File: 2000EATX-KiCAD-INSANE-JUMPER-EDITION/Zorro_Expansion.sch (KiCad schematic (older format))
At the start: 111 parts, among them CN601 Amiga-2000-Zorro-Slot, CN602 Amiga-2000-Zorro-Slot, CN603 Amiga-2000-Zorro-Slot, CN604 Amiga-2000-Zorro-Slot, CN605 Amiga-2000-Zorro-Slot, U606 74HCT32

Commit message: Add files via upload
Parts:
- C617, C619, C620, C621, C622, C623, C624, C625, C626, C627, C628, C629, C630, C631, C632, C633, C635, C637, C639, C641, C645, C647, C649, C650, C651, C652, C654, C655, C657, C658, C659, C660, C661, C662, C663, C664, C665, C666, C667, C668, C669, C670, C671, C672, C673, C674, C675: footprint Capacitor_SMD:C_1206_3216Metric -> Capacitor_SMD:C_0805_2012Metric
- R601A1, R601B1, R601C1, R601D1, R601E1, R601F1, R601G1, R601H1, R601I1, R602A1, R602B1, R602C1, R602D1, R602E1, R602F1, R602G1, R602H1, R602I1, R603A1, R603B1, R603C1, R603D1, R603E1, R603F1, R603G1, R603H1, R603I1, R604, R604A1, R604B1, R604C1, R604D1, R604E1, R604F1, R604G1, R604H1, R604I1, R605, R605A1, R605B1, R605C1, R605D1, R605E1, R605F1, R605G1, R605H1, R605I1: footprint Resistor_SMD:R_1206_3216Metric -> Resistor_SMD:R_0805_2012Metric

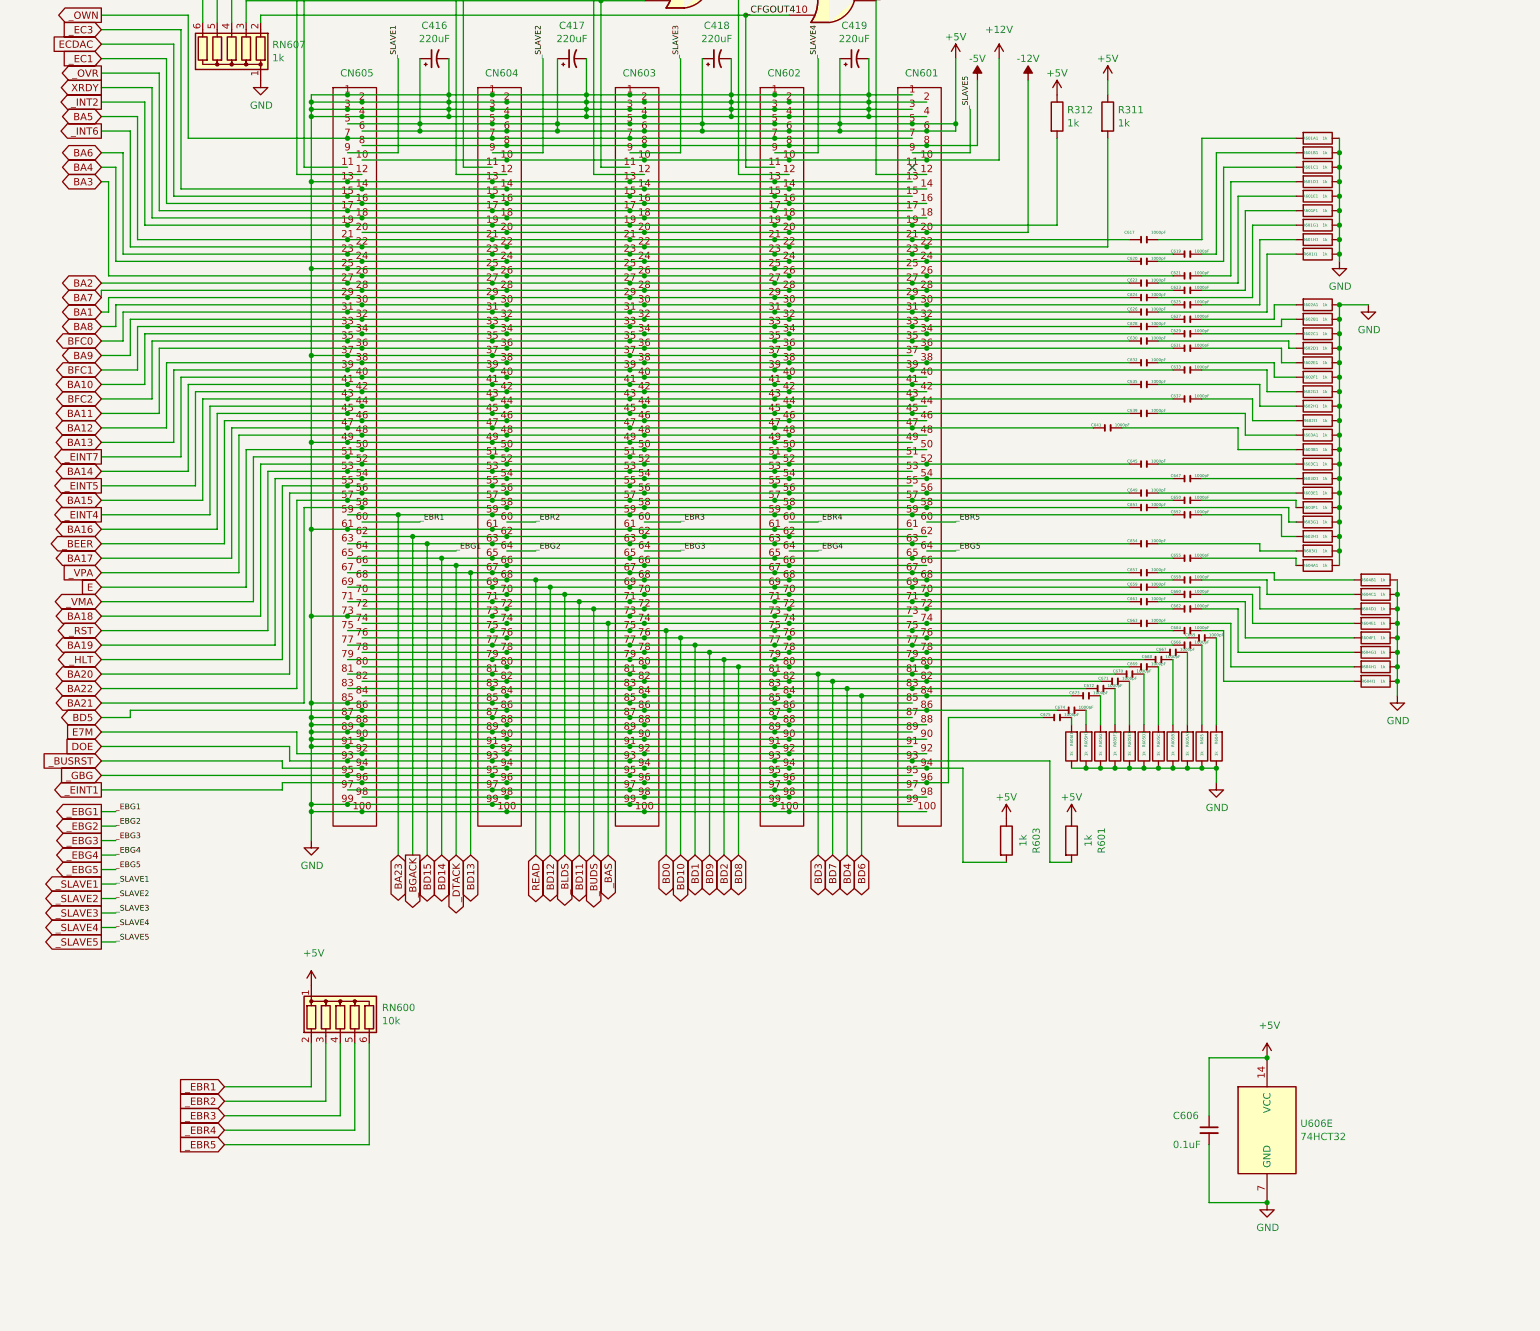
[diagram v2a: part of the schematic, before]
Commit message: Add files via upload
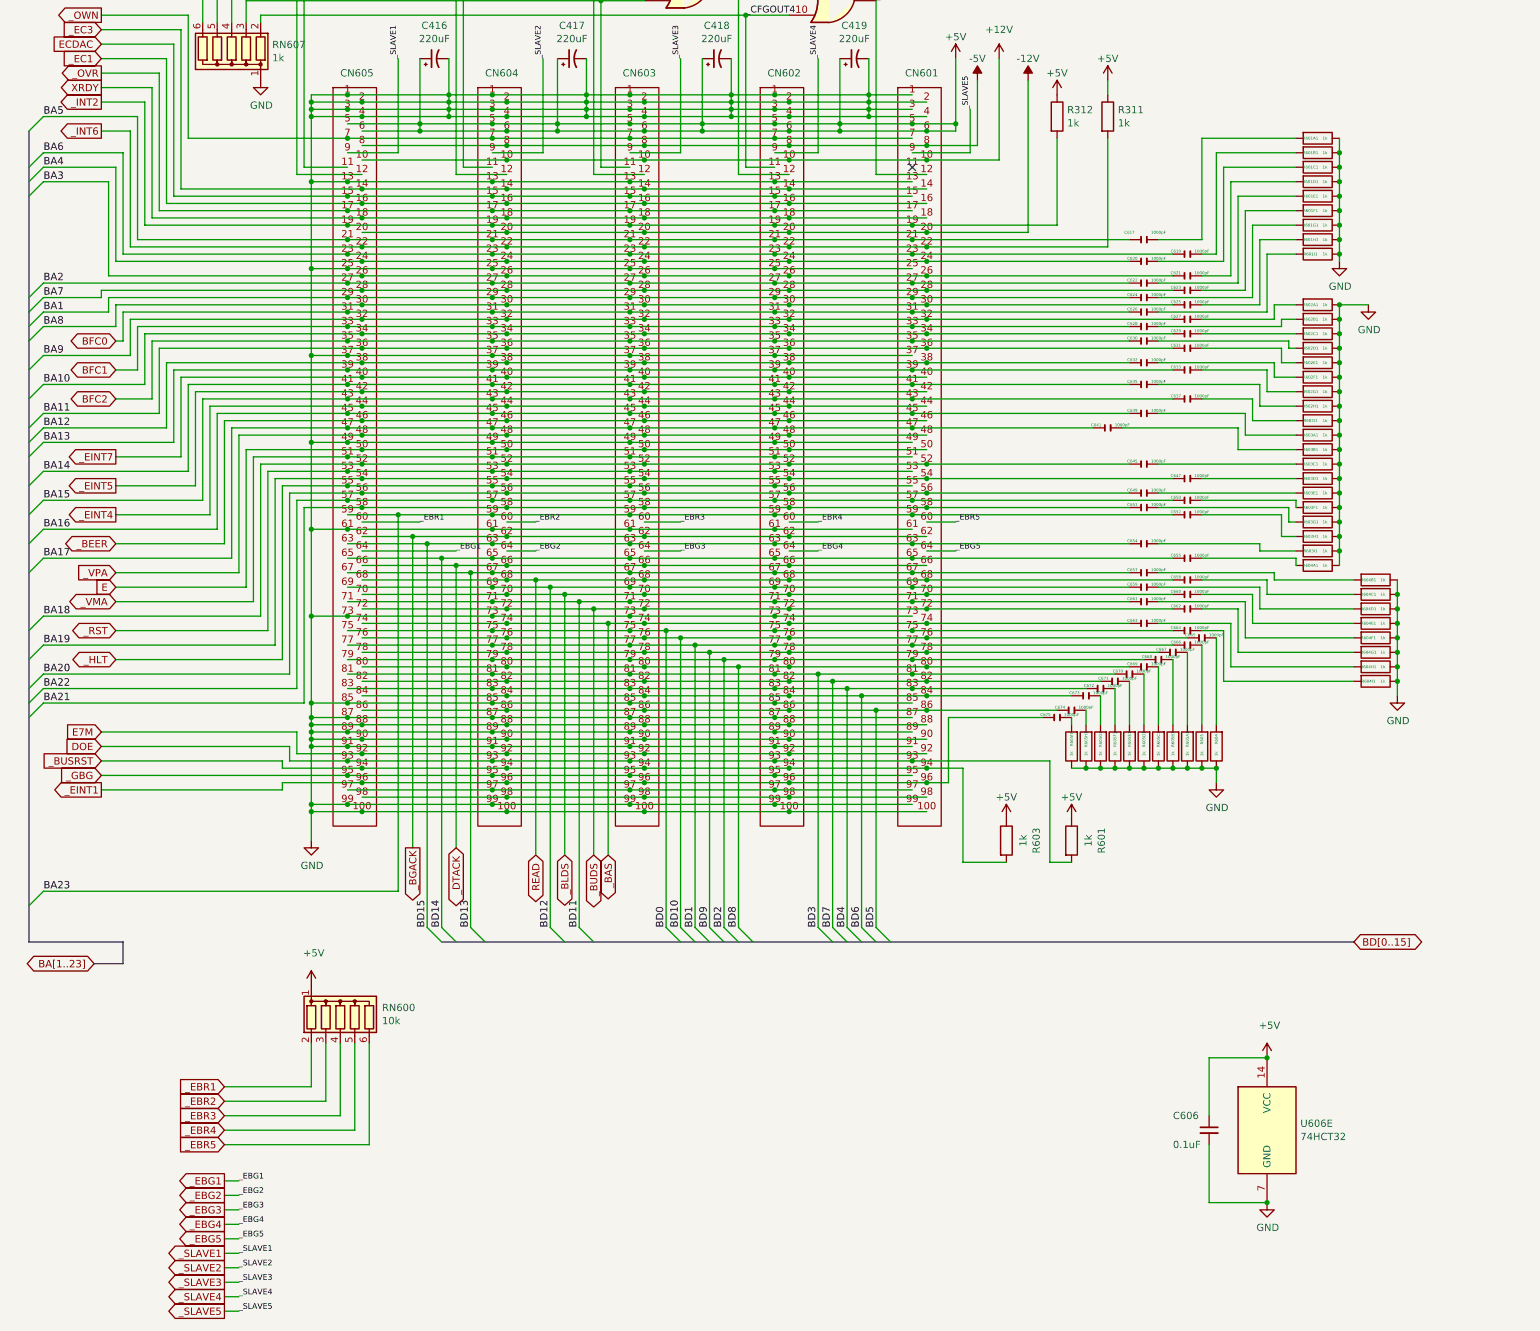
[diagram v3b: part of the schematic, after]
